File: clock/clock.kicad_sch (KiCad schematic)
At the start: 43 parts, among them J1 Conn_01x06, J2 Power_inlet_vertical, J3 Conn_02x03_Odd_Even, J4 Conn_01x05, J5 Conn_01x05, SW1 Omron_B3F_SPST, SW2 Omron_B3F_SPST, SW3 Omron_B3F_SPST, SW4 Omron_B3F_SPST, U1 ATmega328-PU, U2 L7805, U3 MAX7219, U4 DS1307_DIP-8, Y1 Crystal_16MHz, Y2 Crystal_32768Hz

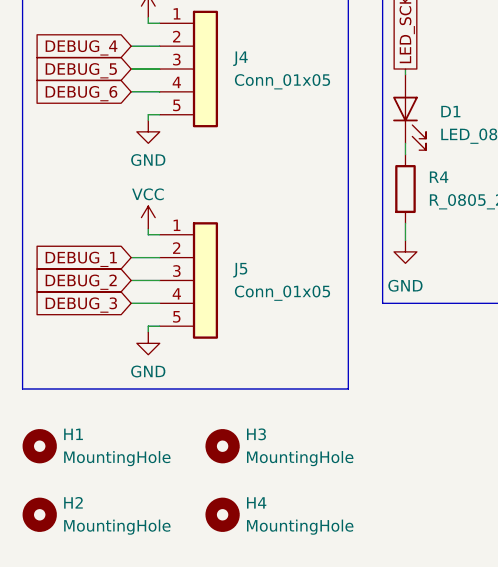
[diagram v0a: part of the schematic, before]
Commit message: lots o' changes
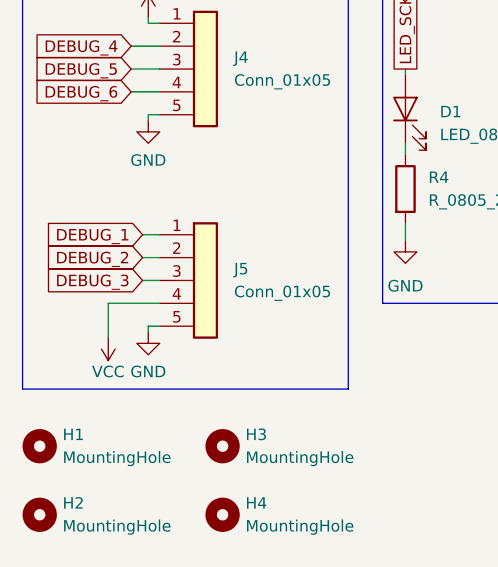
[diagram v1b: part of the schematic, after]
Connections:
- net DEBUG_1: now also J5.1 (Pin_1); no longer J5.2 (Pin_2)
- net DEBUG_2: now also J5.2 (Pin_2); no longer J5.3 (Pin_3)
- net DEBUG_3: now also J5.3 (Pin_3); no longer J5.4 (Pin_4)
- net VCC: now also J5.4 (Pin_4); no longer J5.1 (Pin_1)
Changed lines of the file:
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@@
     (stroke (width 0) (type default) (color 0 0 0 0))
   )
-  (wire (pts (xy 28.575 168.275) (xy 31.75 168.275))
-    (stroke (width 0) (type default) (color 0 0 0 0))
-  )
   (wire (pts (xy 52.07 64.77) (xy 67.31 64.77))
     (stroke (width 0) (type default) (color 0 0 0 0))
@@
     (stroke (width 0) (type default) (color 0 0 0 0))
   )
-  (wire (pts (xy 30.48 171.45) (xy 30.48 170.815))
-    (stroke (width 0) (type default) (color 0 0 0 0))
-  )
   (wire (pts (xy 89.535 82.55) (xy 95.25 82.55))
     (stroke (width 0) (type default) (color 0 0 0 0))
@@
     (stroke (width 0) (type default) (color 0 0 0 0))
   )
+  (wire (pts (xy 26.035 172.085) (xy 26.035 168.275))
+    (stroke (width 0) (type default) (color 0 0 0 0))
+  )
   (wire (pts (xy 226.695 81.28) (xy 281.305 81.28))
     (stroke (width 0) (type default) (color 0 0 0 0))
@@
     (stroke (width 0) (type default) (color 0 0 0 0))
   )
+  (wire (pts (xy 30.48 170.815) (xy 30.48 171.45))
+    (stroke (width 0) (type default) (color 0 0 0 0))
+  )
   (wire (pts (xy 59.055 150.495) (xy 59.055 151.765))
     (stroke (width 0) (type default) (color 0 0 0 0))
@@
     (stroke (width 0) (type default) (color 0 0 0 0))
   )
+  (wire (pts (xy 29.845 163.195) (xy 31.75 163.195))
+    (stroke (width 0) (type default) (color 0 0 0 0))
+  )
   (wire (pts (xy 132.715 182.245) (xy 133.35 182.245))
     (stroke (width 0) (type default) (color 0 0 0 0))
@@
     (stroke (width 0) (type default) (color 0 0 0 0))
   )
-  (wire (pts (xy 28.575 165.735) (xy 31.75 165.735))
-    (stroke (width 0) (type default) (color 0 0 0 0))
-  )
   (wire (pts (xy 278.765 78.74) (xy 278.765 65.405))
     (stroke (width 0) (type default) (color 0 0 0 0))
@@
     (stroke (width 0) (type default) (color 0 0 0 0))
   )
+  (wire (pts (xy 31.75 170.815) (xy 30.48 170.815))
+    (stroke (width 0) (type default) (color 0 0 0 0))
+  )
   (wire (pts (xy 280.035 67.945) (xy 275.59 67.945))
     (stroke (width 0) (type default) (color 0 0 0 0))
@@
     (stroke (width 0) (type default) (color 0 0 0 0))
   )
-  (wire (pts (xy 28.575 163.195) (xy 31.75 163.195))
+  (wire (pts (xy 29.845 165.735) (xy 31.75 165.735))
     (stroke (width 0) (type default) (color 0 0 0 0))
   )
@@
     (stroke (width 0) (type default) (color 0 0 0 0))
   )
-  (wire (pts (xy 30.48 160.02) (xy 30.48 160.655))
-    (stroke (width 0) (type default) (color 0 0 0 0))
-  )
   (wire (pts (xy 194.31 45.085) (xy 200.66 45.085))
     (stroke (width 0) (type default) (color 0 0 0 0))
@@
     (stroke (width 0) (type default) (color 0 0 0 0))
   )
-  (wire (pts (xy 30.48 160.655) (xy 31.75 160.655))
-    (stroke (width 0) (type default) (color 0 0 0 0))
-  )
   (wire (pts (xy 36.83 118.11) (xy 36.83 120.65))
     (stroke (width 0) (type default) (color 0 0 0 0))
@@
     (stroke (width 0) (type default) (color 0 0 0 0))
   )
+  (wire (pts (xy 29.845 160.655) (xy 31.75 160.655))
+    (stroke (width 0) (type default) (color 0 0 0 0))
+  )
   (wire (pts (xy 91.44 72.39) (xy 91.44 74.93))
     (stroke (width 0) (type default) (color 0 0 0 0))
@@
     (stroke (width 0) (type default) (color 0 0 0 0))
   )
+  (wire (pts (xy 26.035 168.275) (xy 31.75 168.275))
+    (stroke (width 0) (type default) (color 0 0 0 0))
+  )
   (wire (pts (xy 196.85 83.185) (xy 200.66 83.185))
     (stroke (width 0) (type default) (color 0 0 0 0))
@@
     (stroke (width 0) (type default) (color 0 0 0 0))
   )
-  (wire (pts (xy 30.48 170.815) (xy 31.75 170.815))
-    (stroke (width 0) (type default) (color 0 0 0 0))
-  )
   (polyline (pts (xy 106.68 88.9) (xy 187.96 88.9))
     (stroke (width 0) (type default) (color 0 0 0 0))
@@
     )
   )
-  (global_label "DEBUG_2" (shape input) (at 28.575 165.735 180) (fields_autoplaced)
+  (global_label "DEBUG_2" (shape input) (at 29.845 163.195 180) (fields_autoplaced)
     (effects (font (size 1.27 1.27)) (justify right))
-    (property "Intersheet References" "${INTERSHEET_REFS}" (id 0) (at 17.6952 165.6556 0)
+    (property "Intersheet References" "${INTERSHEET_REFS}" (id 0) (at 18.9652 163.1156 0)
       (effects (font (size 1.27 1.27)) (justify right) hide)
     )
@@
     )
   )
-  (global_label "DEBUG_1" (shape input) (at 28.575 163.195 180) (fields_autoplaced)
+  (global_label "DEBUG_1" (shape input) (at 29.845 160.655 180) (fields_autoplaced)
     (effects (font (size 1.27 1.27)) (justify right))
-    (property "Intersheet References" "${INTERSHEET_REFS}" (id 0) (at 17.6952 163.1156 0)
+    (property "Intersheet References" "${INTERSHEET_REFS}" (id 0) (at 18.9652 160.5756 0)
       (effects (font (size 1.27 1.27)) (justify right) hide)
     )
@@
     )
   )
-  (global_label "DEBUG_3" (shape input) (at 28.575 168.275 180) (fields_autoplaced)
+  (global_label "DEBUG_3" (shape input) (at 29.845 165.735 180) (fields_autoplaced)
     (effects (font (size 1.27 1.27)) (justify right))
-    (property "Intersheet References" "${INTERSHEET_REFS}" (id 0) (at 17.6952 168.1956 0)
+    (property "Intersheet References" "${INTERSHEET_REFS}" (id 0) (at 18.9652 165.6556 0)
       (effects (font (size 1.27 1.27)) (justify right) hide)
     )
@@
     (pin "1")
   )
-  (symbol (lib_id "HPS:VCC") (at 30.48 160.02 0) (unit 1)
-    (in_bom yes) (on_board yes)
-    (property "Reference" "#PWR032" (id 0) (at 30.48 163.83 0)
-      (effects (font (size 1.27 1.27)) hide)
-    )
-    (property "Value" "VCC" (id 1) (at 30.48 156.21 0))
-    (property "Footprint" "" (id 2) (at 30.48 160.02 0)
-      (effects (font (size 1.27 1.27)) hide)
-    )
-    (property "Datasheet" "" (id 3) (at 30.48 160.02 0)
-      (effects (font (size 1.27 1.27)) hide)
-    )
-    (pin "1")
-  )
   (symbol (lib_id "power:GND") (at 36.83 120.65 0) (unit 1)
     (in_bom yes) (on_board yes) (fields_autoplaced)
@@
     (pin "1")
   )
+  (symbol (lib_id "HPS:GND") (at 30.48 171.45 0) (unit 1)
+    (in_bom yes) (on_board yes)
+    (property "Reference" "#PWR0102" (id 0) (at 30.48 177.8 0)
+      (effects (font (size 1.27 1.27)) hide)
+    )
+    (property "Value" "GND" (id 1) (at 30.48 175.895 0))
+    (property "Footprint" "" (id 2) (at 30.48 171.45 0)
+      (effects (font (size 1.27 1.27)) hide)
+    )
+    (property "Datasheet" "" (id 3) (at 30.48 171.45 0)
+      (effects (font (size 1.27 1.27)) hide)
+    )
+    (pin "1")
+  )
   (symbol (lib_id "HPS:GND") (at 205.74 143.51 0) (unit 1)
     (in_bom yes) (on_board yes) (fields_autoplaced)
@@
     (pin "1")
   )
+  (symbol (lib_id "HPS:VCC") (at 26.035 172.085 180) (unit 1)
+    (in_bom yes) (on_board yes)
+    (property "Reference" "#PWR0101" (id 0) (at 26.035 168.275 0)
+      (effects (font (size 1.27 1.27)) hide)
+    )
+    (property "Value" "VCC" (id 1) (at 26.035 175.895 0))
+    (property "Footprint" "" (id 2) (at 26.035 172.085 0)
+      (effects (font (size 1.27 1.27)) hide)
+    )
+    (property "Datasheet" "" (id 3) (at 26.035 172.085 0)
+      (effects (font (size 1.27 1.27)) hide)
+    )
+    (pin "1")
+  )
   (symbol (lib_id "HPS:GND") (at 130.175 114.3 0) (unit 1)
     (in_bom yes) (on_board yes) (fields_autoplaced)
@@
     (pin "1")
   )
-  (symbol (lib_id "HPS:GND") (at 30.48 171.45 0) (unit 1)
-    (in_bom yes) (on_board yes)
-    (property "Reference" "#PWR033" (id 0) (at 30.48 177.8 0)
-      (effects (font (size 1.27 1.27)) hide)
-    )
-    (property "Value" "GND" (id 1) (at 30.48 175.895 0))
-    (property "Footprint" "" (id 2) (at 30.48 171.45 0)
-      (effects (font (size 1.27 1.27)) hide)
-    )
-    (property "Datasheet" "" (id 3) (at 30.48 171.45 0)
-      (effects (font (size 1.27 1.27)) hide)
-    )
-    (pin "1")
-  )
   (symbol (lib_id "power:GND") (at 208.28 95.885 0) (unit 1)
     (in_bom yes) (on_board yes) (fields_autoplaced)
@@
       (reference "#PWR031") (unit 1) (value "GND") (footprint "")
     )
-    (path "/5ca2aff5-8428-4ced-b68a-5aeac63943f8"
-      (reference "#PWR032") (unit 1) (value "VCC") (footprint "")
+    (path "/c223ef97-abf1-430e-a5cb-a66689c9af56"
+      (reference "#PWR0101") (unit 1) (value "VCC") (footprint "")
     )
-    (path "/f7928c1b-1afb-4ec5-aef6-4935c5e5cb8b"
-      (reference "#PWR033") (unit 1) (value "GND") (footprint "")
+    (path "/80bf18b2-8009-4386-bcfc-e25f03f6c7ef"
+      (reference "#PWR0102") (unit 1) (value "GND") (footprint "")
     )
     (path "/8c33e279-28d8-480f-bd32-b858d3bc749f"
